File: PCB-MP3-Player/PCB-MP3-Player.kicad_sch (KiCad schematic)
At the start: 9 parts, among them J1 Conn_01x02_Pin, J2 PCM5102A, J3 Oled, J4 Conn_01x06_Pin

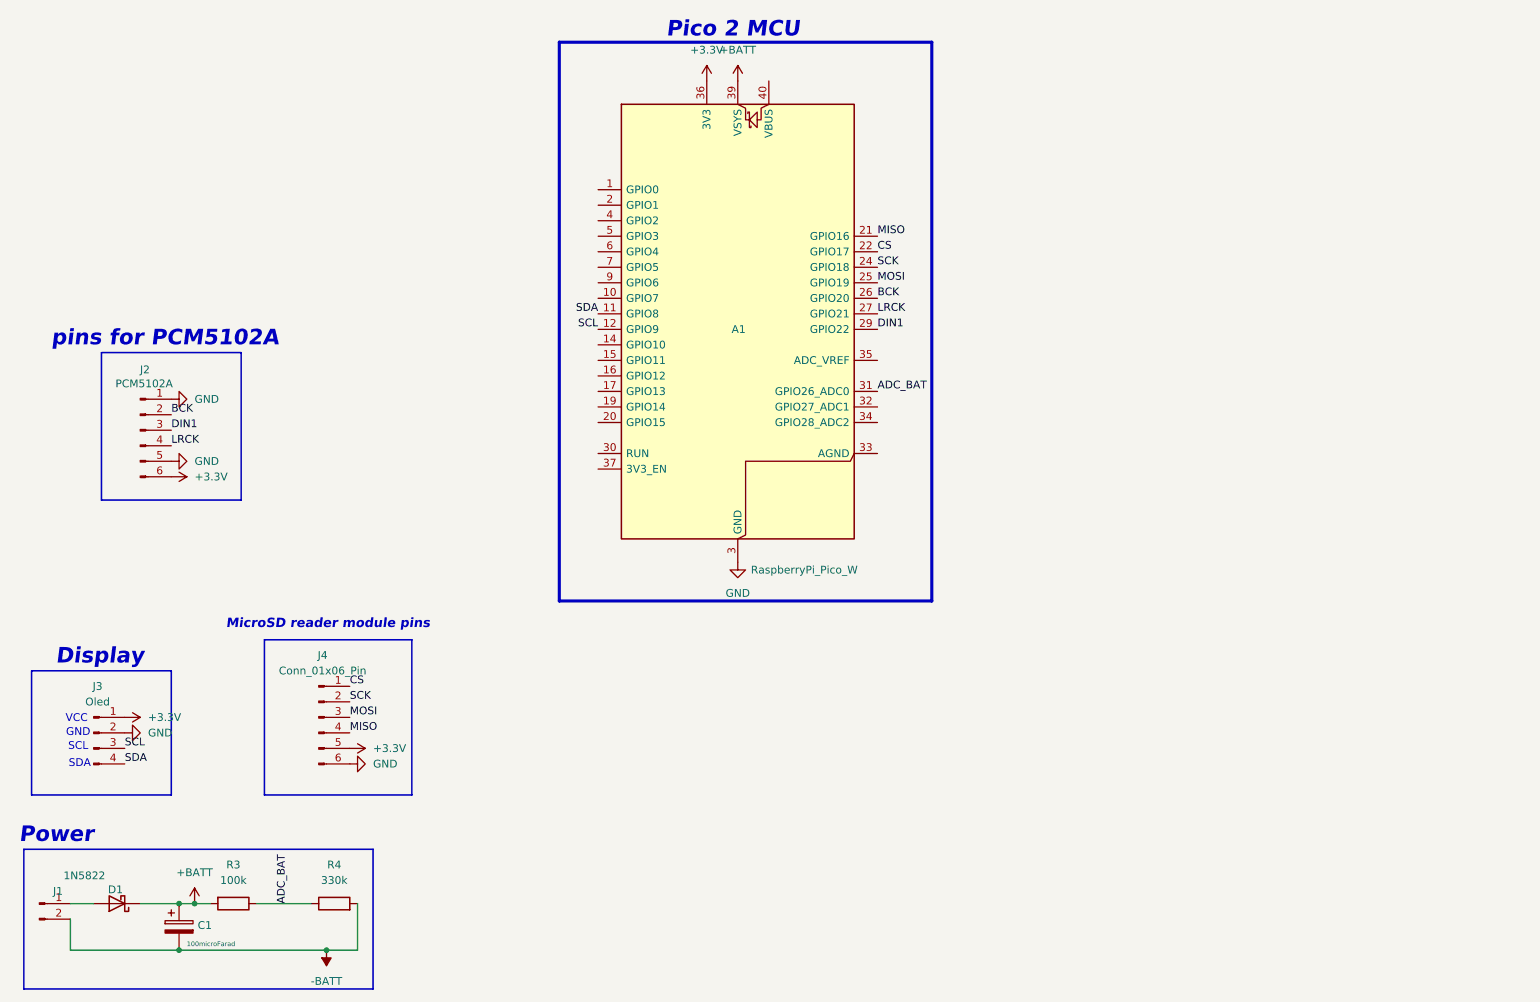
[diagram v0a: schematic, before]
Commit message: pcb changes
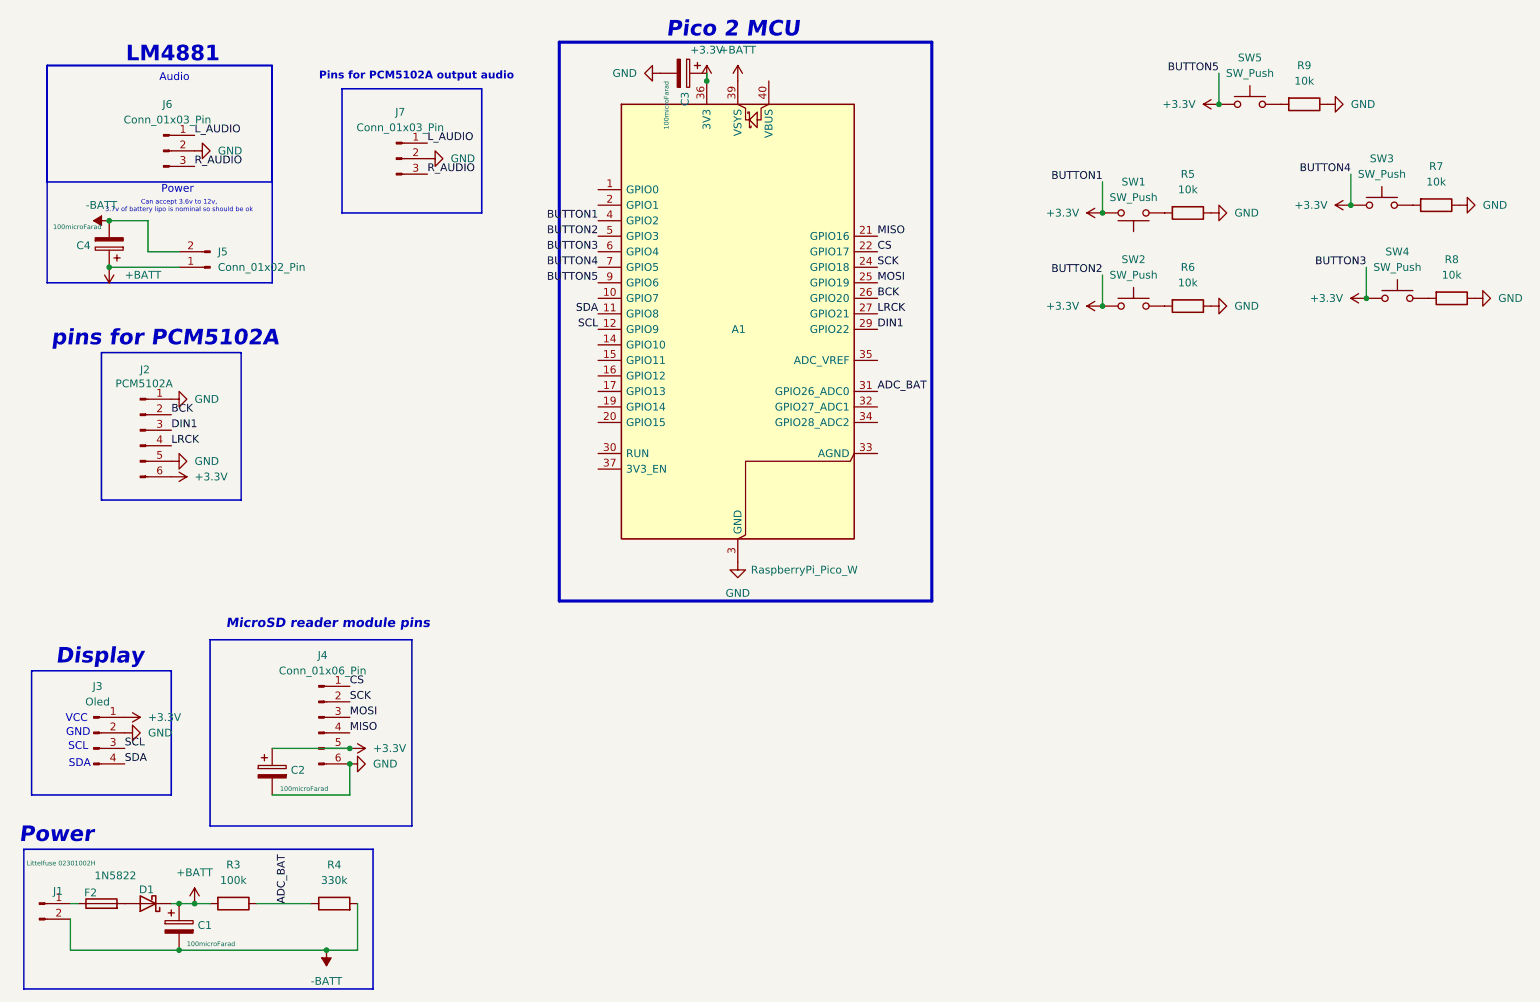
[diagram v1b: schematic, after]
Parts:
- added C2, C3, C4: 100microFarad, Capacitor_THT:CP_Radial_D6.3mm_P2.50mm, symbol Device:C_Polarized
- added F2: Littelfuse 02301002H, Fuse:Fuseholder_Cylinder-5x20mm_Schurter_0031_8201_Horizontal_Open, symbol Device:Fuse
- added J5: Conn_01x02_Pin, Connector_PinSocket_2.54mm:PinSocket_1x02_P2.54mm_Vertical, symbol Connector:Conn_01x02_Pin
- added J6, J7: Conn_01x03_Pin, Connector_PinSocket_2.54mm:PinSocket_1x03_P2.54mm_Vertical, symbol Connector:Conn_01x03_Pin
- added R5, R6, R7, R8, R9: 10k, Resistor_THT:R_Axial_DIN0207_L6.3mm_D2.5mm_P7.62mm_Horizontal, symbol Device:R
- added SW1, SW2, SW3, SW4, SW5: SW_Push, Button_Switch_THT:SW_PUSH_6mm_H4.3mm, symbol Switch:SW_Push
- J4: footprint (none) -> Connector_PinSocket_2.54mm:PinSocket_1x06_P2.54mm_Vertical
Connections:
- net +3.3V: now also A1.4 (GPIO2), A1.5 (GPIO3), A1.6 (GPIO4), A1.7 (GPIO5), A1.9 (GPIO6), C2.1, C3.1, SW1.2, SW2.1, SW3.1, SW4.1, SW5.1
- net +BATT: now also C4.1, J5.1 (Pin_1)
- net -BATT: now also C4.2, J5.2 (Pin_2)
- net GND: now also C2.2, C3.2, J6.2 (Pin_2), J7.2 (Pin_2), R5.1, R6.1, R7.1, R8.1, R9.1
- net at J1.1 (Pin_1): now also F2.1; no longer D1.2 (A)
- new net: R6.2, SW2.2
- new net: R7.2, SW3.2
- new net: R5.2, SW1.1
- new net: R8.2, SW4.2
- new net: D1.2 (A), F2.2
- new net: R9.2, SW5.2
- new net L_AUDIO: J6.1 (Pin_1), J7.1 (Pin_1)
- new net R_AUDIO: J6.3 (Pin_3), J7.3 (Pin_3)
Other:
- note added: "Audio"
- note added: "Can accept 3.6v to 12v, 3.7v of battery lipo is nominal so should be ok"
- note added: "LM4881"
- note added: "Pins for PCM5102A output audio"
- moved on the sheet: D1
